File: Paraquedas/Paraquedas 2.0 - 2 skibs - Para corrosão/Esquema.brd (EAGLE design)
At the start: 51 x 57 mm, 13 parts, among them Q1 IRF540, Q2 IRF540, Q3 IRF540

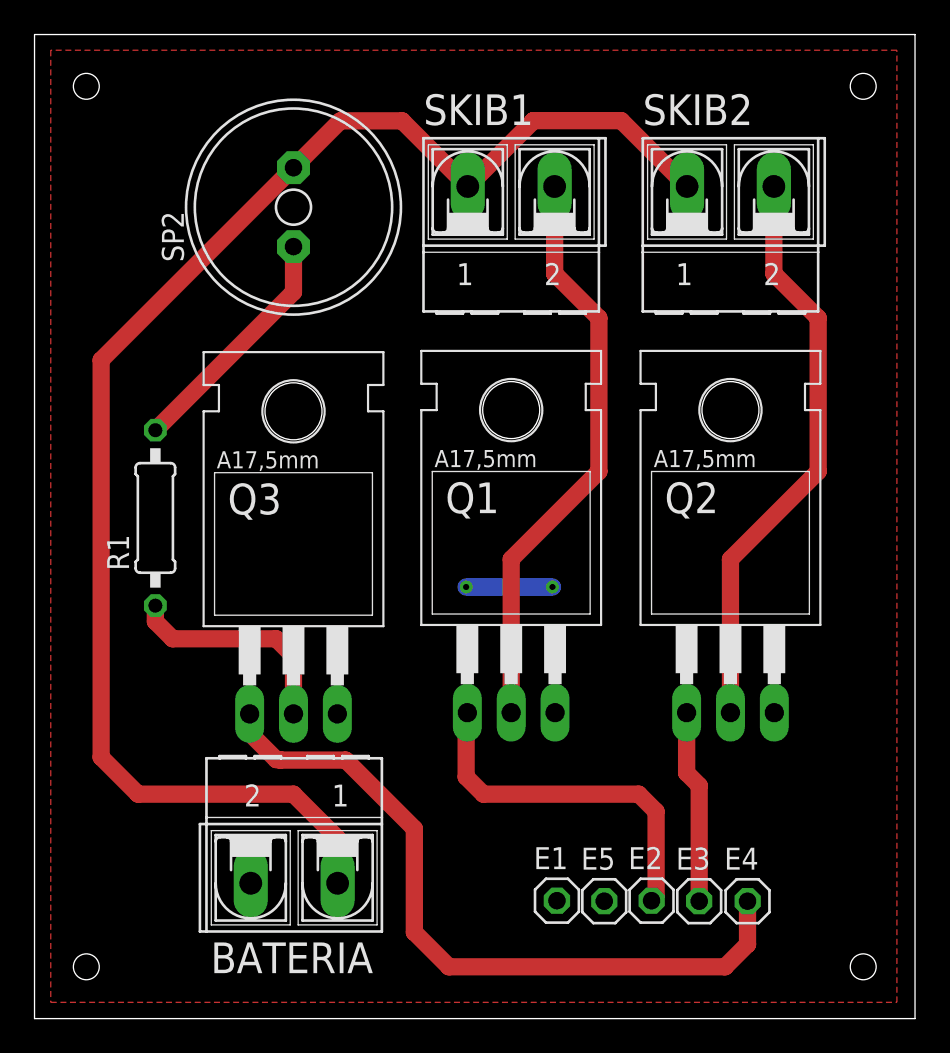
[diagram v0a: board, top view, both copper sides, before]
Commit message: Atualizando placas
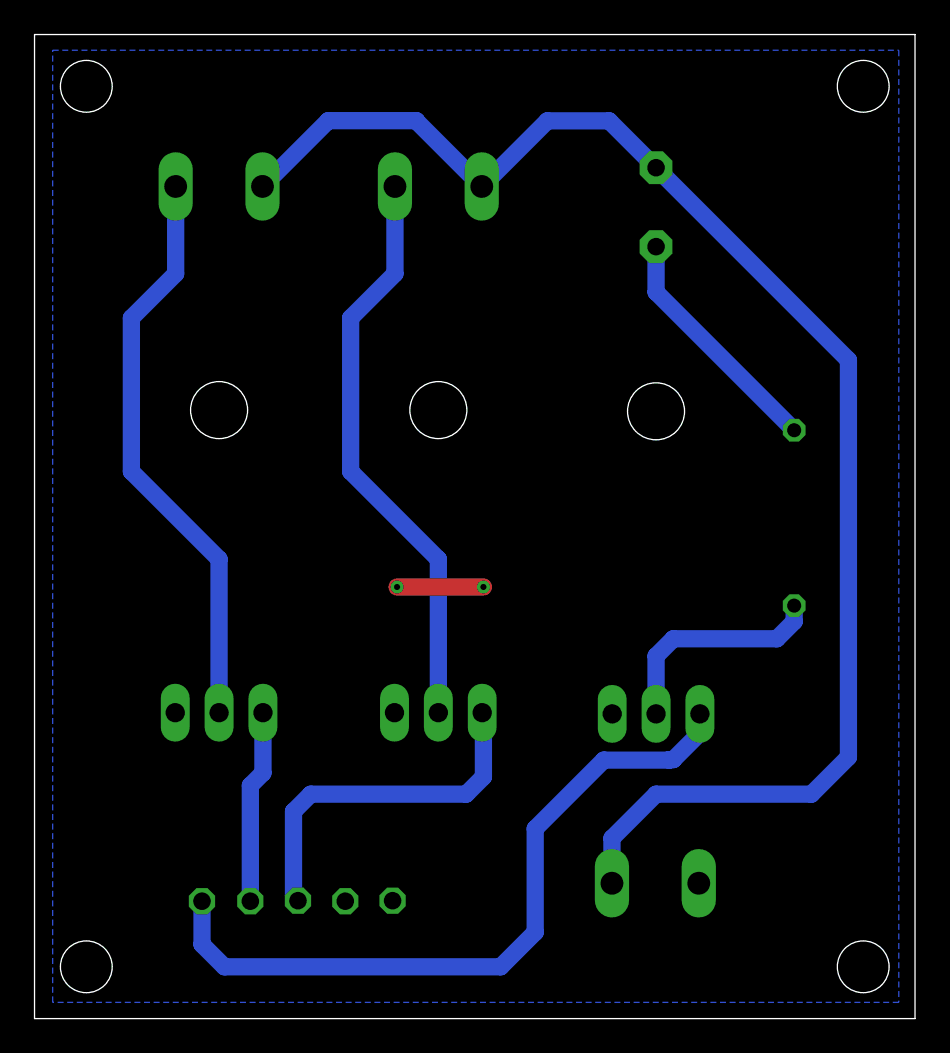
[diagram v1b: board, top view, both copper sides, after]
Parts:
- moved R1 37.0 mm to (43.0, 26.0), flipped to the bottom
- moved E4 31.6 mm to (8.70, 3.80), flipped to the bottom
- moved Q2 29.6 mm to (9.69, 21.1), flipped to the bottom
- moved SKIB2 29.6 mm to (9.69, 45.2), flipped to the bottom
- moved E3 26.0 mm to (11.5, 3.80), flipped to the bottom
- moved Q3 21.0 mm to (35.0, 21.0), flipped to the bottom
- moved SP2 21.0 mm to (35.0, 44.0), flipped to the bottom
- moved BATERIA 20.9 mm to (35.0, 4.84), flipped to the bottom
- moved E2 20.5 mm to (14.3, 3.83), flipped to the bottom
- moved E5 15.0 mm to (17.0, 3.80), flipped to the bottom
- moved E1 9.52 mm to (19.7, 3.83), flipped to the bottom
- moved Q1 4.22 mm to (22.4, 21.1), flipped to the bottom
- moved SKIB1 4.22 mm to (22.4, 45.2), flipped to the bottom
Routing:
- added copper zone on layer 16, net GND
- removed copper zone on layer 1, net GND
